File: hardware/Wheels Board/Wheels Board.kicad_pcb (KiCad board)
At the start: 2 copper layers, 53.6 x 50.5 mm, 44 parts, among them J1 Conn_01x05, J2 Conn_01x05, J4 53307-2471, J5 MX150_02x02_Vertical, U1 ASM330LHHTR, U2 XIAO-ESP32-S3-SMD, U3 TLV9001IDCK, U4 TPS5405DR

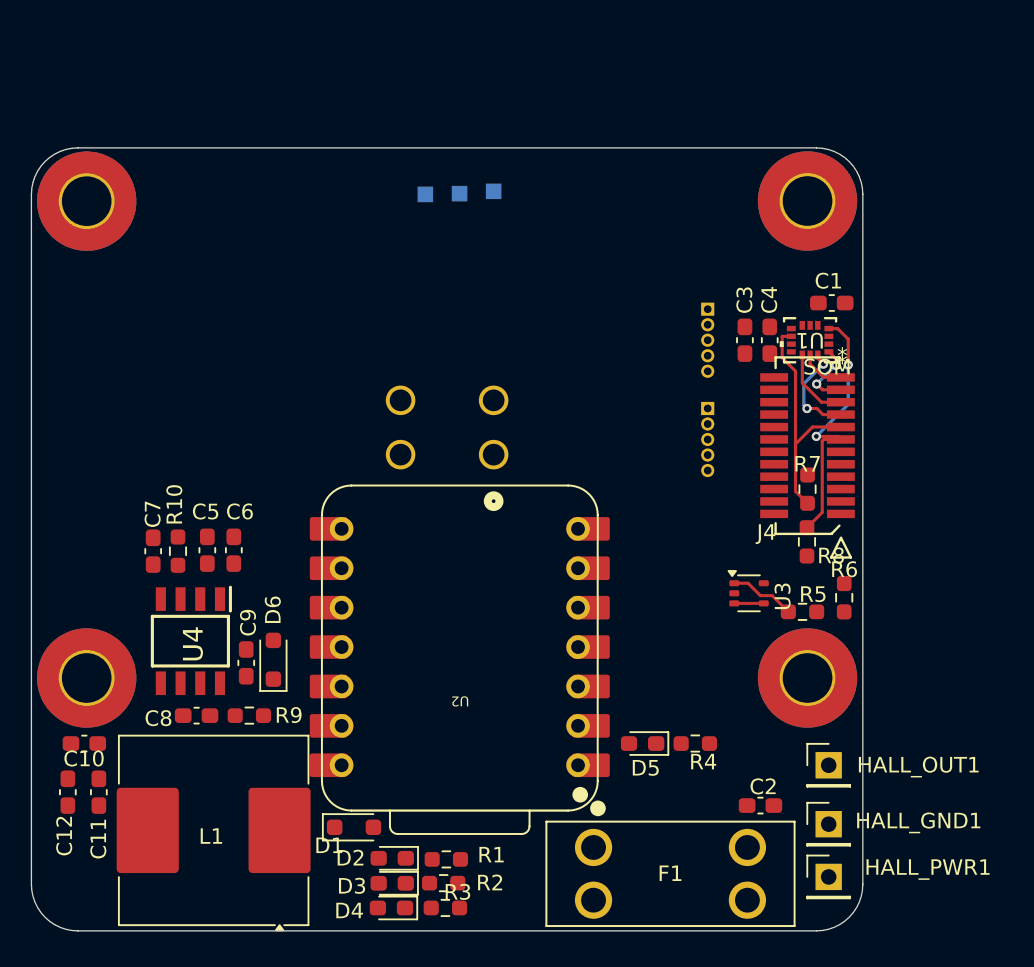
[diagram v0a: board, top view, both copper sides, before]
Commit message: revised layout
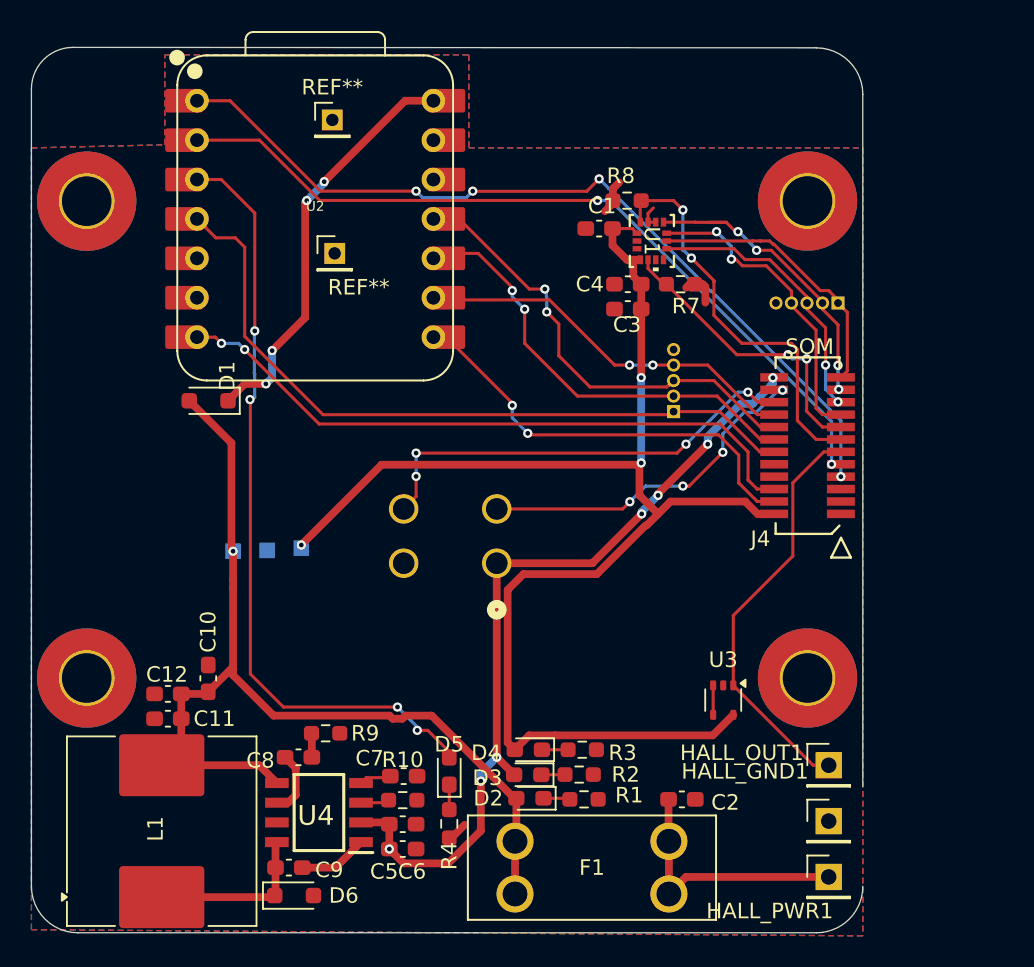
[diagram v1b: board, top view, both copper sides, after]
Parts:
- removed R5: 10k, Resistor_SMD:R_0603_1608Metric_Pad0.98x0.95mm_HandSolder
- removed R6: 19k, Resistor_SMD:R_0603_1608Metric_Pad0.98x0.95mm_HandSolder
- added REF**: PinHeader_1x01_P2.00mm_Vertical, Connector_PinHeader_2.00mm:PinHeader_1x01_P2.00mm_Vertical, F.Cu at (98.4, 61.4)
- added REF**: PinHeader_1x01_P2.00mm_Vertical, Connector_PinHeader_2.00mm:PinHeader_1x01_P2.00mm_Vertical, F.Cu at (98.5, 70.0)
- moved U2 29.1 mm to (97.3, 67.8), turned to 0 degrees
- moved D1 29.1 mm to (90.4, 79.5), turned to 180 degrees
- moved TP_5V1 26.1 mm to (92.0, 89.2)
- moved TP_3.1 26.1 mm to (96.4, 89.0)
- moved TP_GND1 26.1 mm to (94.2, 89.2)
- moved R8 24.9 mm to (117.4, 66.6), turned to 180 degrees
- moved C6 22.1 mm to (102.9, 108.4), turned to 0 degrees
- moved C7 21.7 mm to (103.0, 103.7), turned to 0 degrees
- moved C5 21.7 mm to (102.9, 106.8), turned to 0 degrees
- moved R10 21.6 mm to (102.9, 105.2), turned to 0 degrees
- moved R4 16.7 mm to (105.9, 106.8), turned to -90 degrees
- moved C1 15.7 mm to (115.6, 68.4), turned to 180 degrees
- moved R7 15.5 mm to (120.8, 72.0), turned to 0 degrees
- moved D6 15.3 mm to (95.9, 111.4), turned to 0 degrees
- moved U4 13.8 mm to (97.5, 106.0), turned to 180 degrees
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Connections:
- J1 pad 2: /ESP_SPI_CLK -> /ESP_SPI_MISO
- J1 pad 4: /ESP_SPI_MISO -> /ESP_SPI_CLK
- J2 pad 1: /IMU_SPI_SS -> /IMU_SPI_CLK
- J2 pad 2: /IMU_SPI_CLK -> /IMU_SPI_MISO
- J2 pad 3: /IMU_SPI_MOSI -> /IMU_SPI_SS
- J2 pad 4: /IMU_SPI_MISO -> /IMU_SPI_MOSI
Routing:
- net +3.3V: track 0.00 -> 91.2 mm, vias 0 -> 3
- net +5V: track 0.00 -> 63.9 mm, vias 0 -> 1
- net /EXTRA_GPIO1: track 0.00 -> 54.7 mm, vias 0 -> 4
- net +24V: track 0.00 -> 53.3 mm, vias 0 -> 7
- net /EXTRA_GPIO2: track 0.00 -> 52.0 mm, vias 0 -> 2
- net /XIAO_HEARTBEAT_LED: track 0.00 -> 50.0 mm, vias 0 -> 4
- net /ESP_SPI_SS: track 0.00 -> 47.0 mm
- net /ESP_UART_TX: track 0.00 -> 42.3 mm, vias 0 -> 2
- net /ESP_SPI_MOSI: track 0.00 -> 29.3 mm, vias 0 -> 2
- net /CAN_L: track 0.00 -> 28.9 mm, vias 0 -> 4
- net /ESP_SPI_MISO: track 0.00 -> 27.9 mm, vias 0 -> 2
- net /ESP_UART_RX: track 0.00 -> 27.1 mm, vias 0 -> 2
- net Net-(D1-K): track 0.00 -> 26.8 mm, vias 0 -> 4
- net /ESP_SPI_CLK: track 0.00 -> 24.3 mm, vias 0 -> 2
- net /CAN_H: track 0.00 -> 22.8 mm, vias 0 -> 4
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- added copper zone on B.Cu, net GND
- added copper zone on F.Cu, net GND
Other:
- board size 53.6 x 50.5 mm -> 53.6 x 57.1 mm
- board text added: "SOM"
